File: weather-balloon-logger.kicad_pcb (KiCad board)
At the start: 2 copper layers, 80 x 78.5 mm, 28 parts, among them J1 Conn_01x02, J2 Conn_01x11, J3 SMA, J4 SMA, J5 Conn_01x02, J6 VHF, J7 HF, Q1 AO3400A, SW1 SPDT, U1 PCF8574T, U2 TC4422AVPA

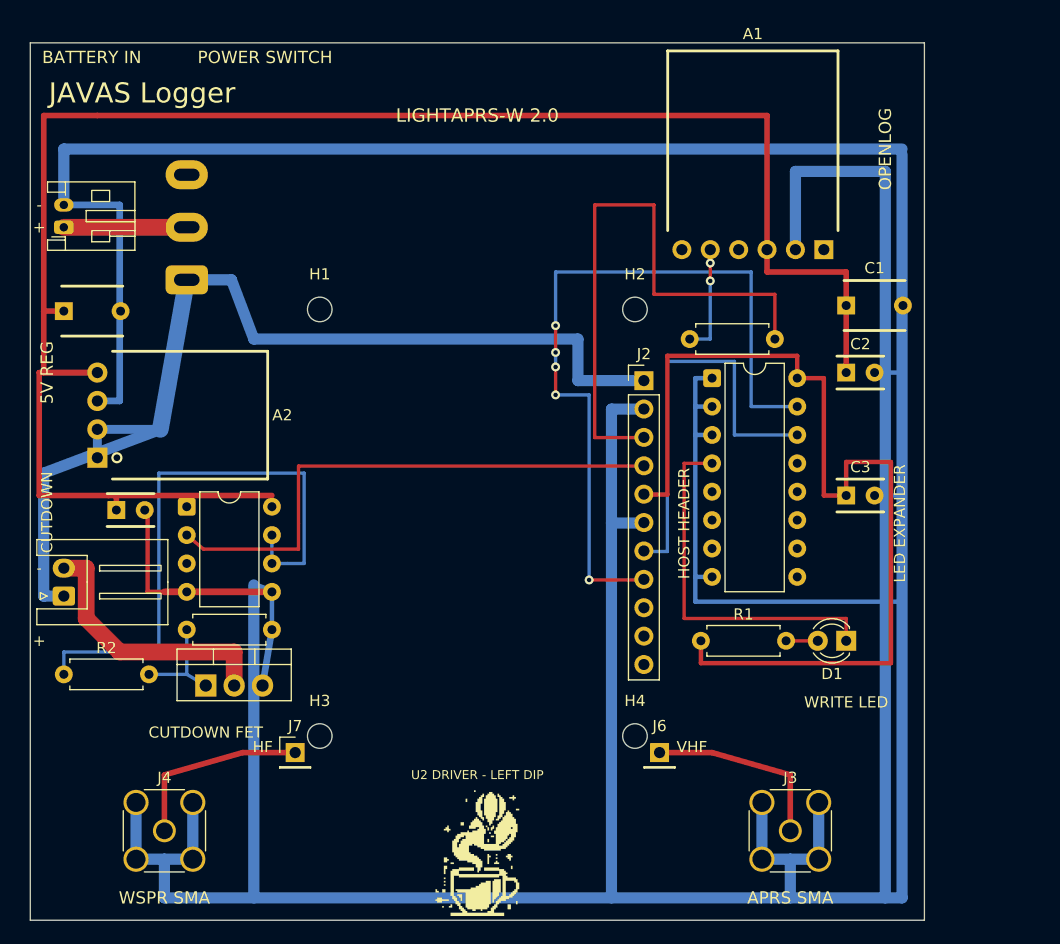
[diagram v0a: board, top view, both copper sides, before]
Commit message: feat(pcb): rebuild for LightHAB
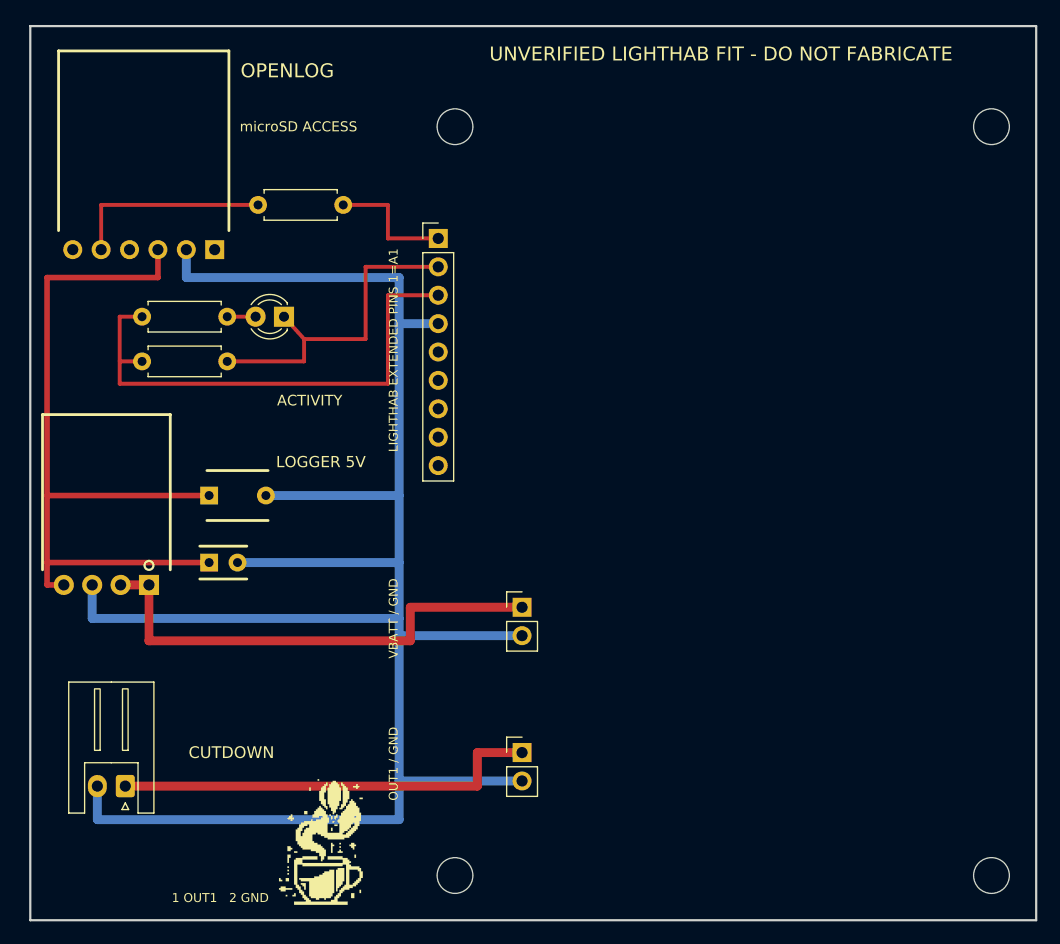
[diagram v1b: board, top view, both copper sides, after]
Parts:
- removed C3, C4: 100nF, KEMET_C315C104K5R5TA
- removed C5: 4.7uF, KEMET_C322C475K5R5TA
- removed J4: SMA, SMA_Amphenol_132134_Vertical
- removed J6: VHF, PinHeader_1x01_P2.54mm_Vertical
- removed J7: HF, PinHeader_1x01_P2.54mm_Vertical
- removed Q1: AO3400A, TO-220-3_Vertical
- removed R3: 1M, R_Axial_DIN0207_L6.3mm_D2.5mm_P7.62mm_Horizontal
- removed SW1: SPDT, SW_CK_7101SYZQE
- removed U1: PCF8574T, DIP-16_W7.62mm
- removed U2: TC4422AVPA, DIP-8_W7.62mm
- D1: value LTST-C190KGKT -> WP710A10SGC
- G1: value Coffee Balloon Logo -> Coffee Balloon
- H1, H2, H3, H4: value M2_STANDOFF -> LIGHTHAB HOLE - UNVERIFIED; footprint MountingHole_2.2mm_M2 -> MountingHole_3.2mm_M3
- J1: value Conn_01x02 -> LightHAB VBATT/GND; footprint JST_PH_S2B-PH-K_1x02_P2.00mm_Horizontal -> PinHeader_1x02_P2.54mm_Vertical
- J2: value Conn_01x11 -> LightHABTracker 1.0; footprint PinHeader_1x11_P2.54mm_Vertical -> PinHeader_1x09_P2.54mm_Vertical
- J3: value SMA -> LightHAB OUT1/GND; footprint SMA_Amphenol_132134_Vertical -> PinHeader_1x02_P2.54mm_Vertical
- J5: value Conn_01x02 -> Cutdown output
- R2: value 100R -> 100k
- moved C1 59.5 mm to (116.0, 132.0)
- moved C2 59.5 mm to (116.0, 138.0)
- moved D1 58.1 mm to (122.7, 116.0)
- moved R1 57.8 mm to (110.0, 116.0)
- moved A1 54.5 mm to (116.5, 110.0)
- moved J1 53.3 mm to (144.0, 142.0), turned to 0 degrees
- moved R4 40.4 mm to (128.0, 106.0)
- moved H2 35.8 mm to (186.0, 99.0)
- moved H4 34.3 mm to (186.0, 166.0)
- moved R2 28.9 mm to (110.0, 120.0)
- moved J3 25.0 mm to (144.0, 155.0)
- moved J2 22.4 mm to (136.5, 109.0)
- moved H1 20.3 mm to (138.0, 99.0)
- moved A2 19.2 mm to (103.0, 140.0), turned to 0 degrees
- moved J5 17.9 mm to (108.5, 158.0), turned to 180 degrees
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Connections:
- A2 pad 1: PACK_SW -> VBATT
- A2 pad 2: PACK_SW -> VBATT
- J1 pad 1: PACK_IN -> VBATT
- J2 pad 1: PACK_SW -> UART_TX
- J2 pad 2: GND -> LED_N
- J2 pad 3: UART_TX -> 3V3
- J2 pad 4: CUTDOWN_CTRL -> GND
- J2 pad 5: 3V3 -> (no net)
- J2 pad 6: GND -> (no net)
- J2 pad 7: I2C_SCL -> (no net)
- J2 pad 8: I2C_SDA -> (no net)
- J3 pad 1: RF_APRS -> OUT1
- J5 pad 1: PACK_SW -> OUT1
- J5 pad 2: CUTDOWN_DRAIN -> GND
- R2 pad 1: CUTDOWN_DRIVE -> 3V3
- R2 pad 2: CUTDOWN_GATE -> LED_N
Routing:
- net GND: track 512.5 -> 182.4 mm
- net PACK_SW: track 94.0 -> 0.00 mm
- net LOGGER_5V: track 162.7 -> 70.4 mm
- net I2C_SDA: track 69.1 -> 0.00 mm, vias 5 -> 0
- net CUTDOWN_DRIVE: track 53.0 -> 0.00 mm
- net CUTDOWN_CTRL: track 48.8 -> 0.00 mm
- net VBATT: track 0.00 -> 43.9 mm
- net UART_TX: track 53.3 -> 11.5 mm
- net 3V3: track 87.0 -> 46.4 mm
- net OUT1: track 0.00 -> 38.5 mm
- net I2C_SCL: track 37.3 -> 0.00 mm
- net CUTDOWN_DRAIN: track 24.0 -> 0.00 mm
- net RF_WSPR: track 17.0 -> 0.00 mm
- net RF_APRS: track 17.0 -> 0.00 mm
- net PACK_IN: track 11.0 -> 0.00 mm
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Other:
- board size 80 x 78.5 mm -> 90 x 80 mm
- board text added: "1 OUT1 2 GND"
- board text added: "ACTIVITY"
- board text added: "COMPONENTS OUT / 18-20mm STACK"
- board text added: "LIGHTHAB 56x75 PHOTO-DERIVED ZONE"
- board text added: "LIGHTHAB EXTENDED PINS 1=A1"
- board text added: "LOGGER 5V"
- board text added: "OUT1 / GND"
- board text added: "SMA KEEP-OUT"
- board text added: "UNVERIFIED LIGHTHAB FIT - DO NOT FABRICATE"
- board text added: "USB KEEP-OUT"
- board text added: "VBATT / GND"
- board text added: "microSD ACCESS"
- board text removed: "+"
- board text removed: "-"
- board text removed: "5V REG"
- board text removed: "APRS 5mm RF CLEARANCE"
- board text removed: "APRS SMA"
- board text removed: "BATTERY IN"
- board text removed: "CUTDOWN FET"
- board text removed: "HF"
- board text removed: "HOST HEADER"
- board text removed: "JAVAS Logger"
- board text removed: "LED EXPANDER"
- board text removed: "LIGHTAPRS-W 2.0"
- board text removed: "LIGHTAPRS-W 2.0 FACE-UP ZONE 32.77 x 54.80 mm"
- board text removed: "POWER SWITCH"
- board text removed: "RESERVED ESD"
- board text removed: "U2 DRIVER - LEFT DIP"
- board text removed: "VHF"
- board text removed: "WRITE LED"
- board text removed: "WSPR 5mm RF CLEARANCE"
- board text removed: "WSPR SMA"
